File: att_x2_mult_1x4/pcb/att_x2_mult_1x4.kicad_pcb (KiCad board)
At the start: 2 copper layers, 17.8 x 102.9 mm, 15 parts, among them J1 AudioJack2_SwitchT, J10 AudioJack2_SwitchT, J2 AudioJack2_SwitchT, J3 AudioJack2_SwitchT, J4 AudioJack2_SwitchT, J5 AudioJack2_SwitchT, J6 AudioJack2_SwitchT, J7 AudioJack2_SwitchT, J8 AudioJack2_SwitchT, J9 AudioJack2_SwitchT

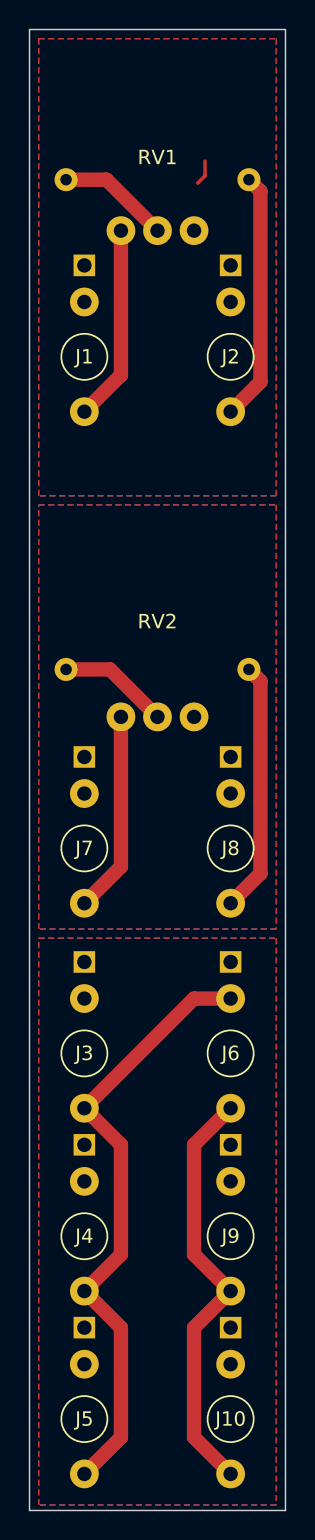
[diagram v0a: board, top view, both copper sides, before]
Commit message: revert cheanges on pat
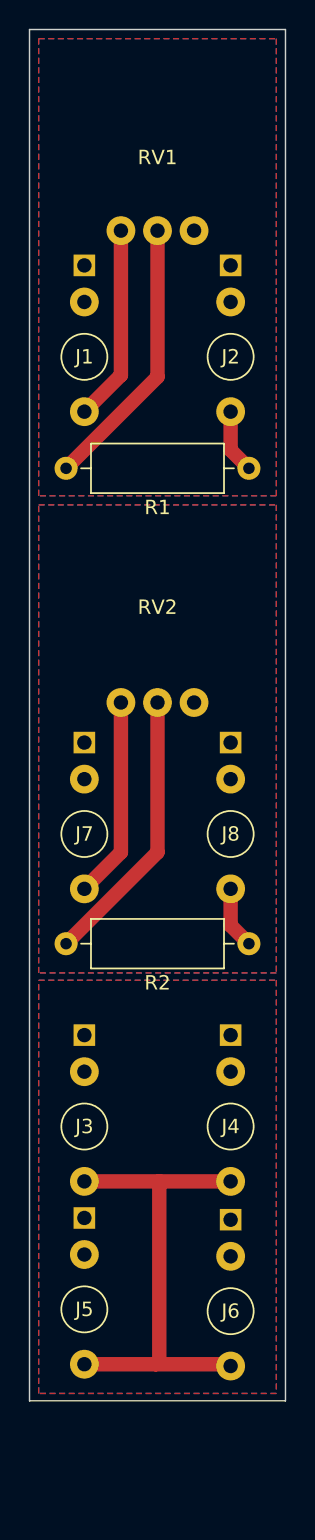
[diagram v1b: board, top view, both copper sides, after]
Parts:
- removed J10, J9: AudioJack2_SwitchT, eurorack_footprints:audio_jack_pj-398sm
- R1, R2: moved to F.Cu
- moved R1 20.0 mm to (108.0, 105.4)
- moved R2 19.1 mm to (108.0, 138.4)
- moved J6 17.9 mm to (106.7, 167.8)
- moved J4 12.7 mm to (106.7, 154.9)
- moved J5 7.62 mm to (96.5, 167.6)
- moved G*** 5.08 mm to (101.6, 151.1)
- moved J3 5.08 mm to (96.5, 154.9)
- moved J7 1.00 mm to (96.5, 134.6)
- moved J8 1.00 mm to (106.7, 134.6)
- moved RV2 1.00 mm to (99.1, 121.7)
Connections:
- J6 pad T: Net-(J10-PadT) -> Net-(J3-PadT)
- J6 pad TN: Net-(J3-PadT) -> unconnected-(J6-PadTN)
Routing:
- net Net-(J10-PadT): track 29.6 -> 0.00 mm
- net Net-(J8-PadT): track 17.4 -> 4.34 mm
- net Net-(J2-PadT): track 17.3 -> 4.46 mm
- net Net-(RV2-Pad2): track 7.72 -> 19.4 mm
- net Net-(RV1-Pad2): track 7.82 -> 19.1 mm
- net Net-(J3-PadT): track 42.9 -> 33.2 mm
- net (no net): track 1.73 -> 0.00 mm
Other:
- board size 17.8 x 102.9 mm -> 17.8 x 95.2 mm
- board text added: "MB20220612"
- board text removed: "MB20220614"
